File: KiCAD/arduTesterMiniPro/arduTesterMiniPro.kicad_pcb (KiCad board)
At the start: 2 copper layers, 123.8 x 57.1 mm, 19 parts, among them J1 3-pin_test_header, J2 3-pin_test_header, J3 2-pin_power_input_header, SW1 SW_Push, U1 LCD_HD44780, U2 Arduino_Mini_Pro

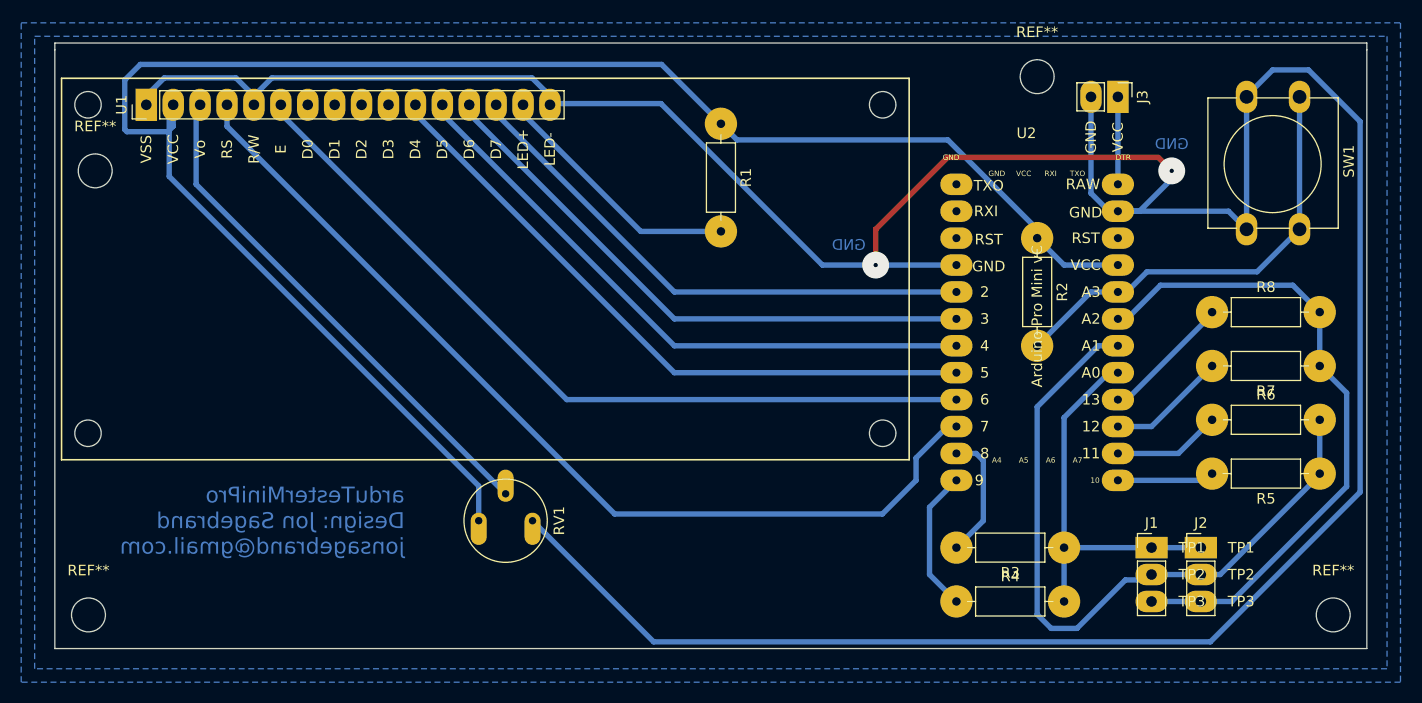
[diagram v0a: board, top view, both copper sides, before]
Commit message: mini pro
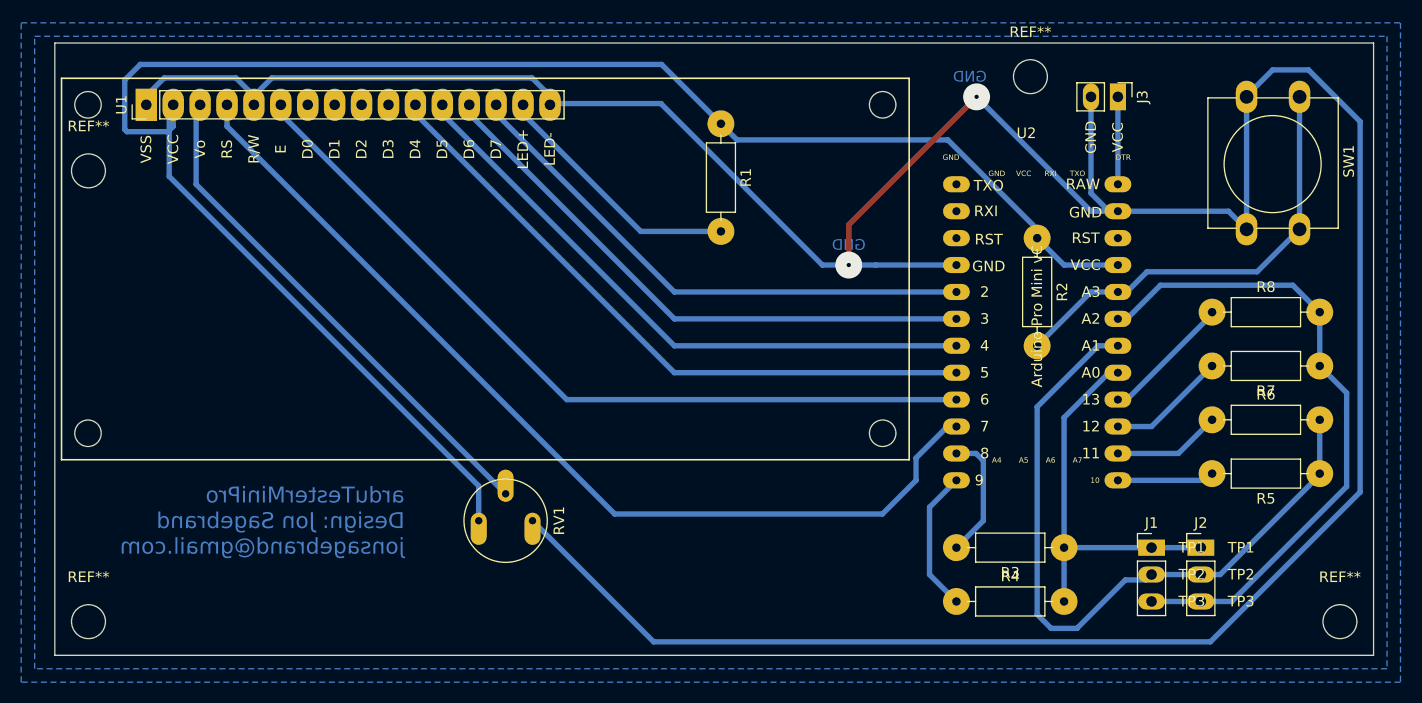
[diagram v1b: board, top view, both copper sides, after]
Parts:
- removed the REF** at (108.6, 71.1)
- removed the REF** at (197.5, 62.2)
- removed the REF** at (225.4, 113.0)
- removed the REF** at (108.0, 113.0)
- added REF**: MountingHole_3.2mm_M3, MountingHole:MountingHole_3.2mm_M3, F.Cu at (108.0, 71.1)
- added REF**: MountingHole_3.2mm_M3, MountingHole:MountingHole_3.2mm_M3, F.Cu at (196.8, 62.2)
- added REF**: MountingHole_3.2mm_M3, MountingHole:MountingHole_3.2mm_M3, F.Cu at (226.1, 113.7)
- added REF**: MountingHole_3.2mm_M3, MountingHole:MountingHole_3.2mm_M3, F.Cu at (108.0, 113.7)
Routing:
- net GND: track 307.6 -> 304.5 mm
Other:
- board size 123.8 x 57.1 mm -> 124.5 x 57.8 mm
- net class Default: clearance 0.762 -> 1.016
- rule trace_clearance: 0.762 -> 1.016
